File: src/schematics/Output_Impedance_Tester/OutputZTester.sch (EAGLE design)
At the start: 108 parts, among them U1 ADG801BRTZ-REEL7, U10 ADG801BRTZ-REEL7, U2 ADA4552-2ARM, U3 ADG801BRTZ-REEL7, U4 ADG801BRTZ-REEL7, U5 ADG801BRTZ-REEL7, U6 ADA4552-2ARM, U7 ADG801BRTZ-REEL7, U8 ADG801BRTZ-REEL7, U9 ADG801BRTZ-REEL7

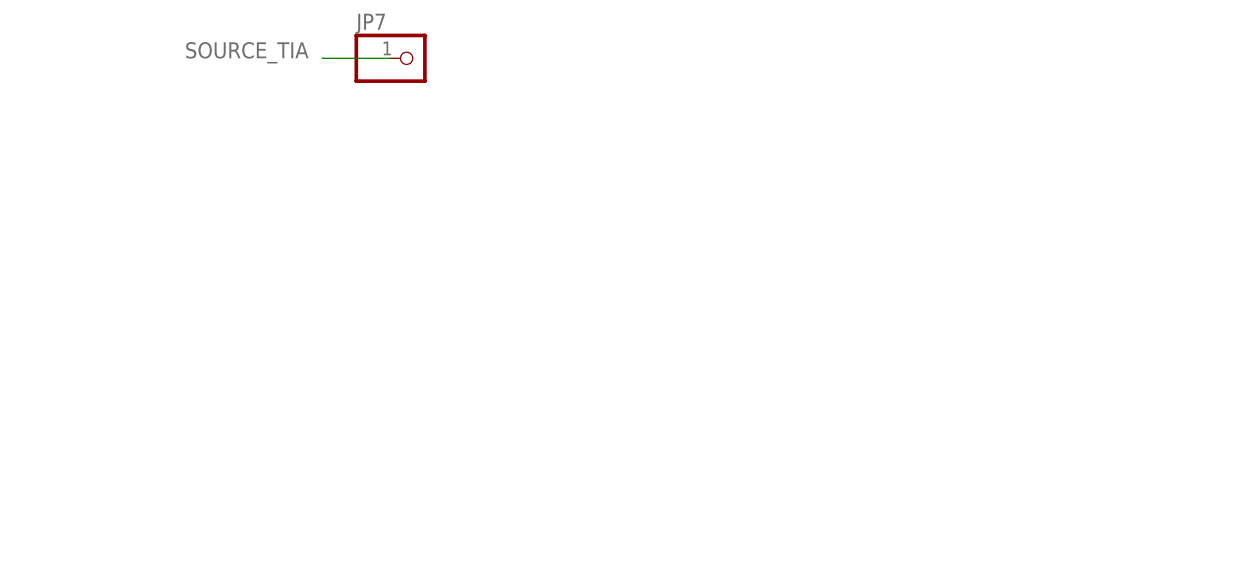
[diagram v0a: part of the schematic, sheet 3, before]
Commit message: one mo' 'gin
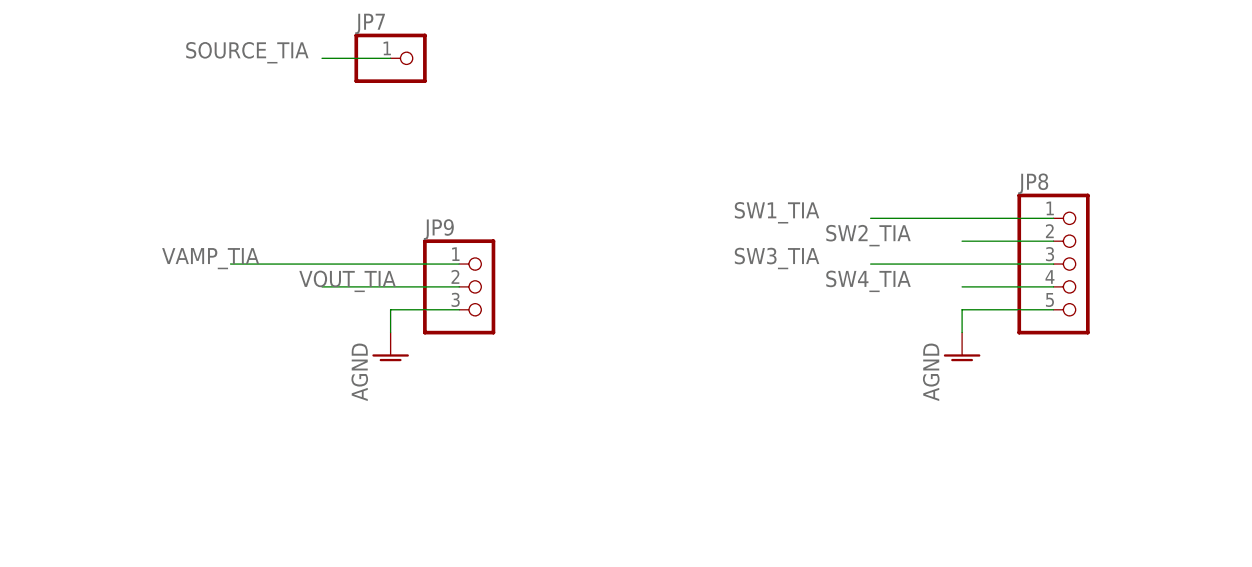
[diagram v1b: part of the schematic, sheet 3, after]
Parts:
- added JP8: (no value), pinhead:PINHD-1X5/90
- added JP9: (no value), pinhead:PINHD-1X3/90
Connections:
- net AGND: now also JP8.5, JP9.3
- net SW1_TIA: now also JP8.1
- net SW2_TIA: now also JP8.2
- net SW3_TIA: now also JP8.3
- net SW4_TIA: now also JP8.4
- net VAMP_TIA: now also JP9.1
- net VOUT_TIA: now also JP9.2
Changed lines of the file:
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@@
 <setting verticaltext="up"/>
 </settings>
-<grid distance="0.1" unitdist="inch" unit="inch" style="lines" multiple="1" display="yes" altdistance="0.01" altunitdist="inch" altunit="inch"/>
+<grid distance="0.1" unitdist="inch" unit="inch" style="lines" multiple="1" display="no" altdistance="0.01" altunitdist="inch" altunit="inch"/>
 <layers>
 <layer number="1" name="Top" color="4" fill="1" visible="no" active="no"/>
@@
 <part name="C19" library="rcl" deviceset="C-EU" device="C0402" value="0.1uF"/>
 <part name="P+13" library="supply1" deviceset="V+" device=""/>
+<part name="JP8" library="pinhead" deviceset="PINHD-1X5" device="/90"/>
+<part name="AGND28" library="supply1" deviceset="AGND" device=""/>
+<part name="JP9" library="pinhead" deviceset="PINHD-1X3" device="/90"/>
+<part name="AGND29" library="supply1" deviceset="AGND" device=""/>
 </parts>
 <sheets>
@@
 <instance part="C19" gate="G$1" x="144.78" y="205.74" rot="R180"/>
 <instance part="P+13" gate="1" x="144.78" y="220.98"/>
+<instance part="JP8" gate="A" x="276.86" y="53.34"/>
+<instance part="AGND28" gate="VR1" x="264.16" y="43.18"/>
+<instance part="JP9" gate="A" x="210.82" y="50.8"/>
+<instance part="AGND29" gate="VR1" x="200.66" y="43.18"/>
 </instances>
 <busses>
@@
 <junction x="160.02" y="198.12"/>
 </segment>
+<segment>
+<pinref part="AGND28" gate="VR1" pin="AGND"/>
+<wire x1="264.16" y1="45.72" x2="264.16" y2="48.26" width="0.1524" layer="91"/>
+<pinref part="JP8" gate="A" pin="5"/>
+<wire x1="264.16" y1="48.26" x2="274.32" y2="48.26" width="0.1524" layer="91"/>
+</segment>
+<segment>
+<pinref part="JP9" gate="A" pin="3"/>
+<wire x1="208.28" y1="48.26" x2="200.66" y2="48.26" width="0.1524" layer="91"/>
+<wire x1="200.66" y1="48.26" x2="200.66" y2="45.72" width="0.1524" layer="91"/>
+<pinref part="AGND29" gate="VR1" pin="AGND"/>
+</segment>
 </net>
 <net name="V-" class="0">
@@
 <label x="144.78" y="76.2" size="1.778" layer="95"/>
 </segment>
+<segment>
+<pinref part="JP9" gate="A" pin="1"/>
+<wire x1="208.28" y1="53.34" x2="182.88" y2="53.34" width="0.1524" layer="91"/>
+<label x="175.26" y="53.34" size="1.778" layer="95"/>
+</segment>
 </net>
 <net name="VOUT_TIA" class="0">
@@
 <label x="45.72" y="78.74" size="1.778" layer="95"/>
 </segment>
+<segment>
+<pinref part="JP9" gate="A" pin="2"/>
+<wire x1="208.28" y1="50.8" x2="193.04" y2="50.8" width="0.1524" layer="91"/>
+<label x="190.5" y="50.8" size="1.778" layer="95"/>
+</segment>
 </net>
 <net name="VLOAD_TIA" class="0">
@@
 <label x="147.32" y="208.28" size="1.778" layer="95"/>
 </segment>
+<segment>
+<pinref part="JP8" gate="A" pin="1"/>
+<wire x1="274.32" y1="58.42" x2="254" y2="58.42" width="0.1524" layer="91"/>
+<label x="238.76" y="58.42" size="1.778" layer="95"/>
+</segment>
 </net>
 <net name="SOURCE_TIA" class="0">
@@
 <label x="147.32" y="127" size="1.778" layer="95"/>
 </segment>
+<segment>
+<pinref part="JP8" gate="A" pin="2"/>
+<wire x1="274.32" y1="55.88" x2="264.16" y2="55.88" width="0.1524" layer="91"/>
+<label x="248.92" y="55.88" size="1.778" layer="95"/>
+</segment>
 </net>
 <net name="SW3_TIA" class="0">
@@
 <label x="246.38" y="124.46" size="1.778" layer="95"/>
 </segment>
+<segment>
+<pinref part="JP8" gate="A" pin="3"/>
+<wire x1="274.32" y1="53.34" x2="254" y2="53.34" width="0.1524" layer="91"/>
+<label x="238.76" y="53.34" size="1.778" layer="95"/>
+</segment>
 </net>
 <net name="SW4_TIA" class="0">
@@
 <label x="337.82" y="124.46" size="1.778" layer="95"/>
 </segment>
-</net>
+<segment>
+<pinref part="JP8" gate="A" pin="4"/>
+<wire x1="274.32" y1="50.8" x2="264.16" y2="50.8" width="0.1524" layer="91"/>
+<label x="248.92" y="50.8" size="1.778" layer="95"/>
+</segment>
+</net>
